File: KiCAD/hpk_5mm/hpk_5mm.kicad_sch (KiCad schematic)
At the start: 11 parts, among them J1 Conn_01x03, J2 Conn_Coaxial, U1 OPA810xDBV

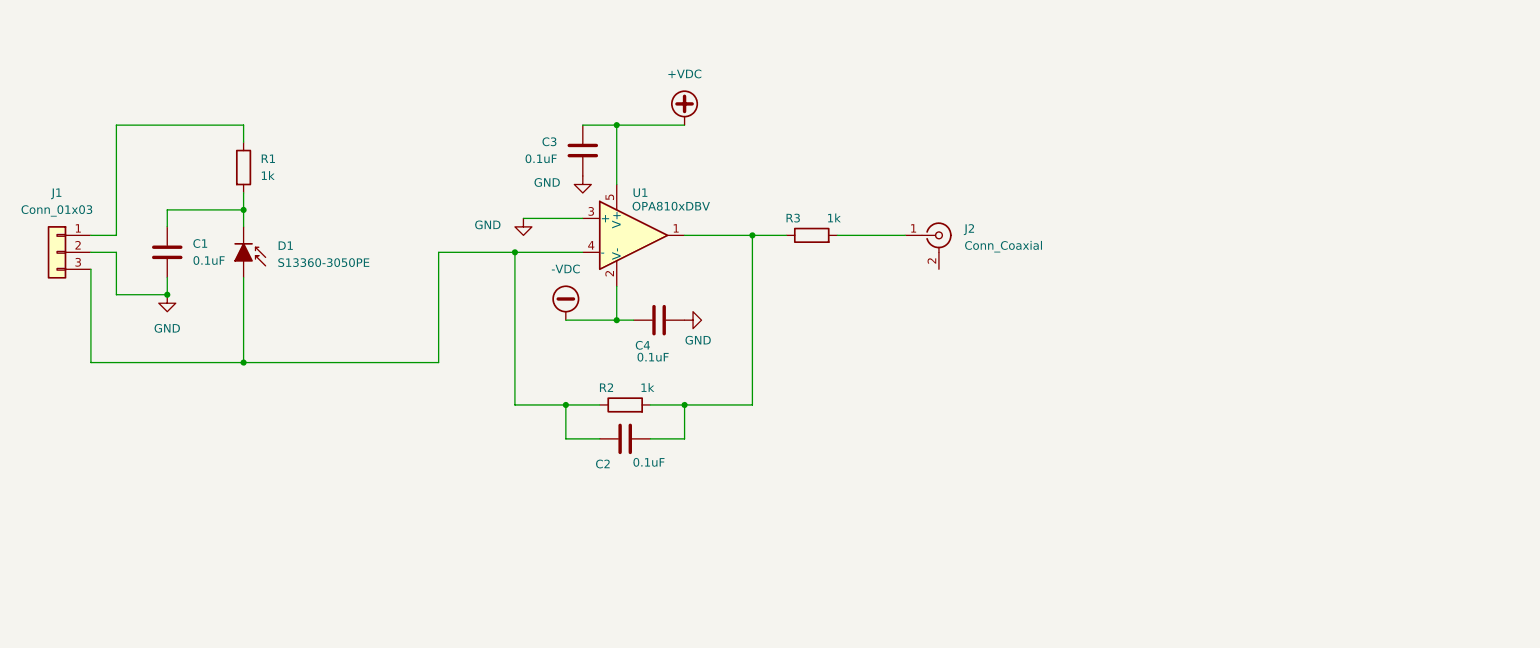
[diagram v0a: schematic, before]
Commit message: trial 3-channel flexi
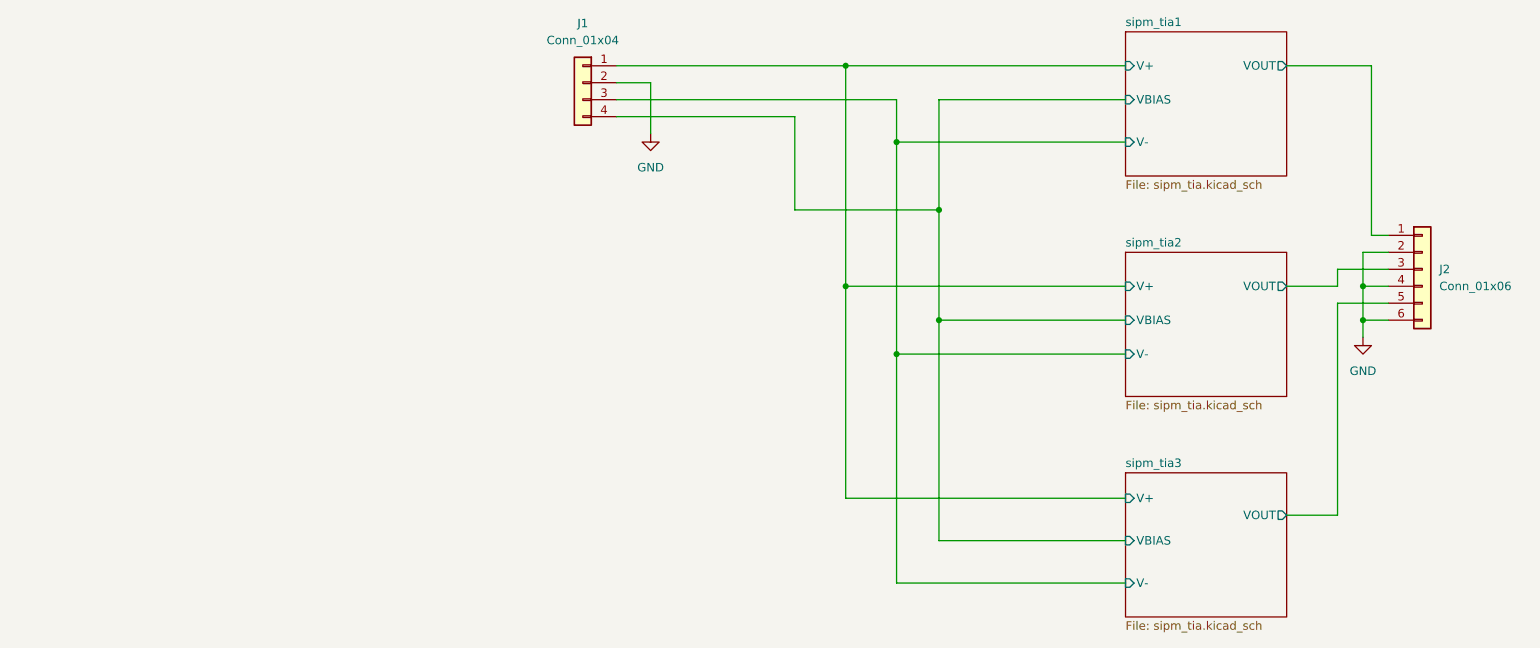
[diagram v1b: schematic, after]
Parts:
- removed C1, C2, C3, C4: 0.1uF, Capacitor_SMD:C_0402_1005Metric, symbol Device:C
- removed D1: S13360-3050PE, my_sipm:s13360-3050pe, symbol Device:D_Photo_Filled
- removed J1: Conn_01x03, Connector_PinHeader_1.00mm:PinHeader_1x03_P1.00mm_Vertical, symbol Connector_Generic:Conn_01x03
- removed J2: Conn_Coaxial, symbol Connector:Conn_Coaxial
- removed R1, R2, R3: 1k, Resistor_SMD:R_0402_1005Metric, symbol Device:R
- removed U1: OPA810xDBV, Package_TO_SOT_SMD:SOT-23-5, symbol Amplifier_Operational:OPA810xDBV
- added J1: Conn_01x04, Connector_PinHeader_1.00mm:PinHeader_1x04_P1.00mm_Vertical, symbol Connector_Generic:Conn_01x04
- added J2: Conn_01x06, Connector_PinHeader_1.00mm:PinHeader_1x06_P1.00mm_Vertical, symbol Connector_Generic:Conn_01x06
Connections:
- net GND: now also J1.2 (Pin_2), J2.2 (Pin_2), J2.4 (Pin_4), J2.6 (Pin_6)
- new net sipm_tia1/V+: J1.1 (Pin_1)
- new net sipm_tia1/V-: J1.3 (Pin_3)
- new net sipm_tia1/VBIAS: J1.4 (Pin_4)
- new net sipm_tia1/VOUT: J2.1 (Pin_1)
- new net sipm_tia2/VOUT: J2.3 (Pin_3)
- new net sipm_tia3/VOUT: J2.5 (Pin_5)
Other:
- added sheet sipm_tia1 (sipm_tia.kicad_sch)
- added sheet sipm_tia2 (sipm_tia.kicad_sch)
- added sheet sipm_tia3 (sipm_tia.kicad_sch)
